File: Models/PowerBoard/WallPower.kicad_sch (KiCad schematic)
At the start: 1 part

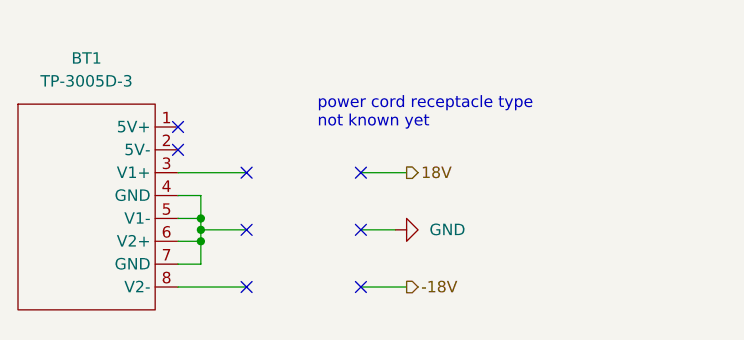
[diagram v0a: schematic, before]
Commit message: Save progress
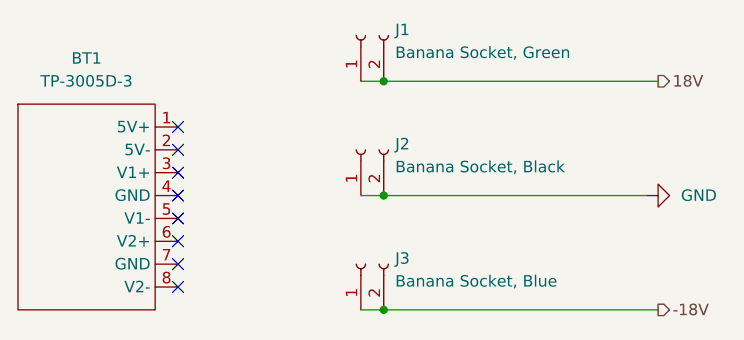
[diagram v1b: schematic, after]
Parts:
- added J1: Banana Socket, Green, symbol Connector:Conn_01x02_Socket
- added J2: Banana Socket, Black, symbol Connector:Conn_01x02_Socket
- added J3: Banana Socket, Blue, symbol Connector:Conn_01x02_Socket
- BT1: now left out of the parts list
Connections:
- net -18V: now also J3.1 (Pin_1), J3.2 (Pin_2)
- net 18V: now also J1.1 (Pin_1), J1.2 (Pin_2)
- net GND: now also J2.1 (Pin_1), J2.2 (Pin_2)
- now unconnected: BT1.4 (GND), BT1.5 (V1-), BT1.6 (V2+), BT1.7 (GND)
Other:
- note removed: "power cord receptacle type not known yet"
